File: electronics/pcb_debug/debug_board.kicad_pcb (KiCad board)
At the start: 2 copper layers, 40.9 x 30.6 mm, 11 parts, among them J1 SWD Device, J2 SWD Probe

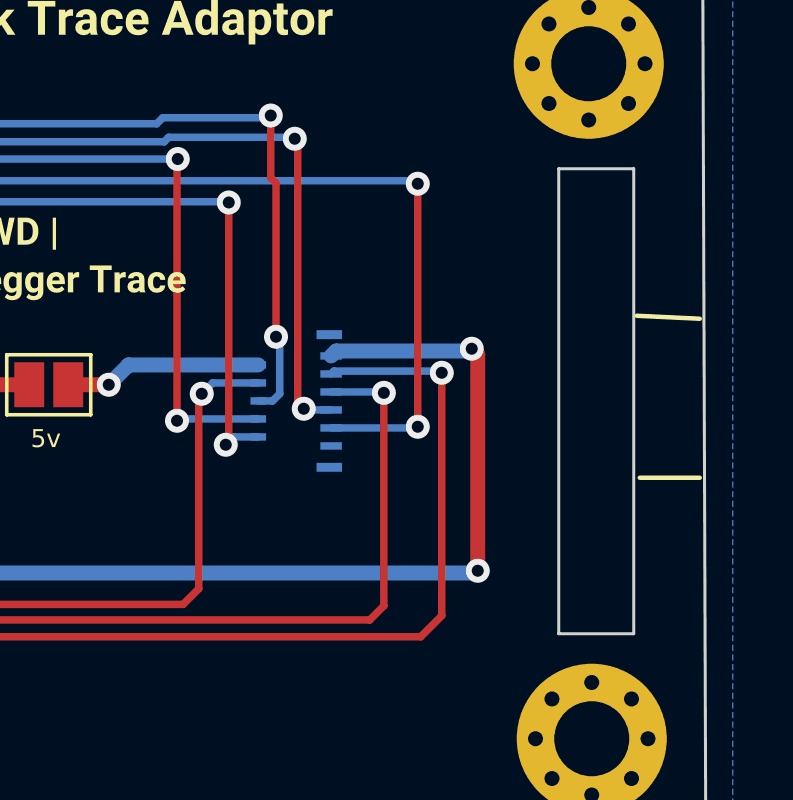
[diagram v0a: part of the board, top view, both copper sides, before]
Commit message: BOM update
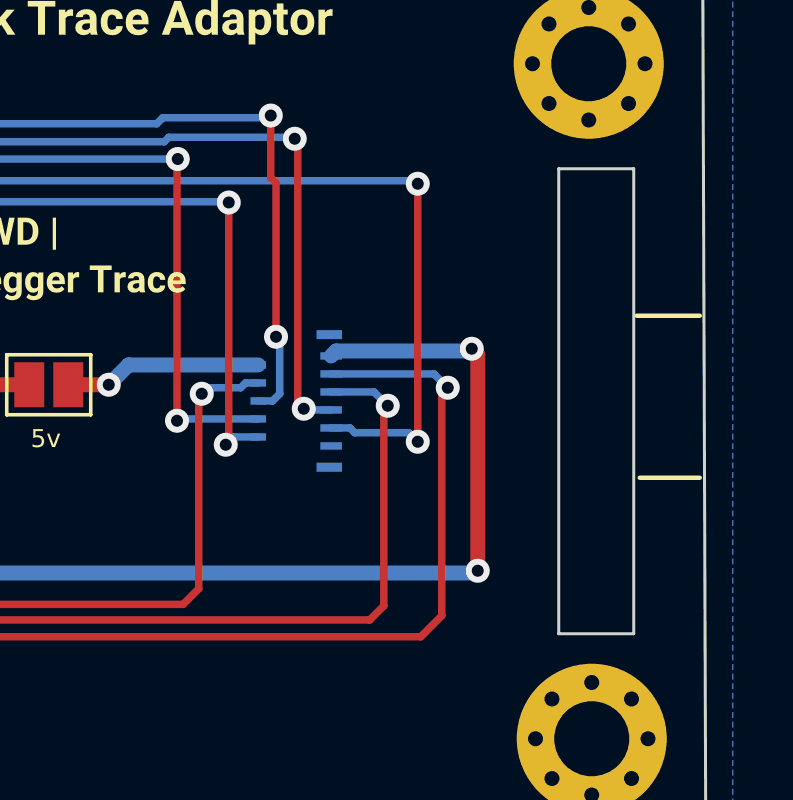
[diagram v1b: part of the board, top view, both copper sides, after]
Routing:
- net /TRACED2: track 33.9 -> 34.6 mm
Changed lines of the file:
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@@
   (gr_circle (center 94.6 65) (end 94.916228 65) (layer "F.SilkS") (width 0.15) (fill solid))
   (gr_rect (start 94 58.2) (end 94.9 60.4) (layer "F.SilkS") (width 0.15) (fill solid))
-  (gr_line (start 119.9 56.5) (end 117.8 56.4) (layer "F.SilkS") (width 0.15))
+  (gr_line (start 119.9 56.4) (end 117.8 56.4) (layer "F.SilkS") (width 0.15))
   (gr_line (start 119.9 61.8) (end 117.9 61.8) (layer "F.SilkS") (width 0.15))
   (gr_line (start 79.207107 44.907107) (end 79.2 73.5) (layer "Edge.Cuts") (width 0.1))
@@
   (segment (start 100.86 58.04) (end 100.2 58.7) (width 0.5) (layer "B.Cu") (net 2))
   (segment (start 105.1835 58.04) (end 100.86 58.04) (width 0.5) (layer "B.Cu") (net 2))
+  (segment (start 89.9 66.2) (end 89.9 60.4) (width 0.25) (layer "F.Cu") (net 3))
+  (segment (start 89.9 60.4) (end 90.405 59.895) (width 0.25) (layer "F.Cu") (net 3))
   (segment (start 90.8 67.1) (end 89.9 66.2) (width 0.25) (layer "F.Cu") (net 3))
-  (segment (start 111.3 58.3) (end 111.3 66.4) (width 0.25) (layer "F.Cu") (net 3))
-  (segment (start 89.9 60.4) (end 90.405 59.895) (width 0.25) (layer "F.Cu") (net 3))
+  (segment (start 111.3 59) (end 111.3 66.4) (width 0.25) (layer "F.Cu") (net 3))
+  (segment (start 111.5 58.8) (end 111.3 59) (width 0.25) (layer "F.Cu") (net 3))
+  (segment (start 111.3 66.4) (end 110.6 67.1) (width 0.25) (layer "F.Cu") (net 3))
   (segment (start 110.6 67.1) (end 90.8 67.1) (width 0.25) (layer "F.Cu") (net 3))
   (segment (start 90.405 59.895) (end 91.555 59.895) (width 0.25) (layer "F.Cu") (net 3))
-  (segment (start 111.3 66.4) (end 110.6 67.1) (width 0.25) (layer "F.Cu") (net 3))
-  (segment (start 89.9 66.2) (end 89.9 60.4) (width 0.25) (layer "F.Cu") (net 3))
-  (via (at 111.3 58.3) (size 0.8) (drill 0.4) (layers "F.Cu" "B.Cu") (net 3))
-  (segment (start 107.6135 58.34) (end 107.708011 58.245489) (width 0.25) (layer "B.Cu") (net 3))
-  (segment (start 107.708011 58.245489) (end 111.245489 58.245489) (width 0.25) (layer "B.Cu") (net 3))
-  (segment (start 111.245489 58.245489) (end 111.3 58.3) (width 0.25) (layer "B.Cu") (net 3))
+  (via (at 111.5 58.8) (size 0.8) (drill 0.4) (layers "F.Cu" "B.Cu") (net 3))
+  (segment (start 111.5 58.8) (end 111.04 58.34) (width 0.25) (layer "B.Cu") (net 3))
+  (segment (start 111.04 58.34) (end 107.6135 58.34) (width 0.25) (layer "B.Cu") (net 3))
   (segment (start 91.92 66.02) (end 91.555 65.655) (width 0.25) (layer "F.Cu") (net 4))
   (segment (start 103.3 59) (end 103.2 59.1) (width 0.25) (layer "F.Cu") (net 4))
@@
   (segment (start 91.555 65.655) (end 91.555 64.975) (width 0.25) (layer "F.Cu") (net 4))
   (via (at 103.3 59) (size 0.8) (drill 0.4) (layers "F.Cu" "B.Cu") (net 4))
-  (segment (start 103.66 58.64) (end 105.1835 58.64) (width 0.25) (layer "B.Cu") (net 4))
-  (segment (start 103.3 59) (end 103.66 58.64) (width 0.25) (layer "B.Cu") (net 4))
+  (segment (start 103.5 58.8) (end 104.598989 58.8) (width 0.25) (layer "B.Cu") (net 4))
+  (segment (start 104.758989 58.64) (end 105.1835 58.64) (width 0.25) (layer "B.Cu") (net 4))
+  (segment (start 103.3 59) (end 103.5 58.8) (width 0.25) (layer "B.Cu") (net 4))
+  (segment (start 104.598989 58.8) (end 104.758989 58.64) (width 0.25) (layer "B.Cu") (net 4))
+  (segment (start 109.5 59.4) (end 109.37 59.53) (width 0.25) (layer "F.Cu") (net 5))
+  (segment (start 91.17952 66.53952) (end 90.46 65.82) (width 0.25) (layer "F.Cu") (net 5))
+  (segment (start 109.37 66.07) (end 108.90048 66.53952) (width 0.25) (layer "F.Cu") (net 5))
+  (segment (start 109.37 59.53) (end 109.37 66.07) (width 0.25) (layer "F.Cu") (net 5))
   (segment (start 90.46 64.19) (end 90.945 63.705) (width 0.25) (layer "F.Cu") (net 5))
-  (segment (start 91.17952 66.53952) (end 90.46 65.82) (width 0.25) (layer "F.Cu") (net 5))
-  (segment (start 109.37 58.97) (end 109.37 66.07) (width 0.25) (layer "F.Cu") (net 5))
   (segment (start 108.90048 66.53952) (end 91.17952 66.53952) (width 0.25) (layer "F.Cu") (net 5))
-  (segment (start 109.37 66.07) (end 108.90048 66.53952) (width 0.25) (layer "F.Cu") (net 5))
+  (segment (start 90.46 65.82) (end 90.46 64.19) (width 0.25) (layer "F.Cu") (net 5))
   (segment (start 90.945 63.705) (end 91.555 63.705) (width 0.25) (layer "F.Cu") (net 5))
-  (segment (start 90.46 65.82) (end 90.46 64.19) (width 0.25) (layer "F.Cu") (net 5))
-  (via (at 109.37 58.97) (size 0.8) (drill 0.4) (layers "F.Cu" "B.Cu") (net 5))
-  (segment (start 107.6135 58.94) (end 109.34 58.94) (width 0.25) (layer "B.Cu") (net 5))
-  (segment (start 109.34 58.94) (end 109.37 58.97) (width 0.25) (layer "B.Cu") (net 5))
+  (via (at 109.5 59.4) (size 0.8) (drill 0.4) (layers "F.Cu" "B.Cu") (net 5))
+  (segment (start 109.04 58.94) (end 107.6135 58.94) (width 0.25) (layer "B.Cu") (net 5))
+  (segment (start 109.5 59.4) (end 109.04 58.94) (width 0.25) (layer "B.Cu") (net 5))
   (segment (start 89.325 58.625) (end 91.555 58.625) (width 0.25) (layer "F.Cu") (net 6))
   (segment (start 105.6 49.726489) (end 105.6 51.8) (width 0.25) (layer "F.Cu") (net 6))
@@
   (segment (start 90.799913 51.175489) (end 102.499989 51.175489) (width 0.25) (layer "B.Cu") (net 8))
   (segment (start 91.100011 51.899989) (end 90.64952 52.35048) (width 0.25) (layer "F.Cu") (net 9))
-  (segment (start 110.5 52) (end 110.5 60.1) (width 0.25) (layer "F.Cu") (net 9))
   (segment (start 90.64952 52.35048) (end 90.64952 53.90952) (width 0.25) (layer "F.Cu") (net 9))
+  (segment (start 110.5 52) (end 110.5 60.6) (width 0.25) (layer "F.Cu") (net 9))
   (segment (start 91.452741 51.899989) (end 91.100011 51.899989) (width 0.25) (layer "F.Cu") (net 9))
   (segment (start 90.64952 53.90952) (end 91.555 54.815) (width 0.25) (layer "F.Cu") (net 9))
-  (via (at 110.5 60.1) (size 0.8) (drill 0.4) (layers "F.Cu" "B.Cu") (net 9))
+  (via (at 110.5 60.6) (size 0.8) (drill 0.4) (layers "F.Cu" "B.Cu") (net 9))
   (via (at 91.452741 51.899989) (size 0.8) (drill 0.4) (layers "F.Cu" "B.Cu") (net 9))
   (via (at 110.5 52) (size 0.8) (drill 0.4) (layers "F.Cu" "B.Cu") (net 9))
+  (segment (start 110.5 60.6) (end 110.2 60.3) (width 0.25) (layer "B.Cu") (net 9))
   (segment (start 110.4 51.9) (end 110.5 52) (width 0.25) (layer "B.Cu") (net 9))
-  (segment (start 110.46 60.14) (end 107.6135 60.14) (width 0.25) (layer "B.Cu") (net 9))
   (segment (start 91.452741 51.899989) (end 91.452752 51.9) (width 0.25) (layer "B.Cu") (net 9))
   (segment (start 91.452752 51.9) (end 110.4 51.9) (width 0.25) (layer "B.Cu") (net 9))
-  (segment (start 110.5 60.1) (end 110.46 60.14) (width 0.25) (layer "B.Cu") (net 9))
+  (segment (start 108.24 60.14) (end 107.6135 60.14) (width 0.25) (layer "B.Cu") (net 9))
+  (segment (start 108.4 60.3) (end 108.24 60.14) (width 0.25) (layer "B.Cu") (net 9))
+  (segment (start 110.2 60.3) (end 108.4 60.3) (width 0.25) (layer "B.Cu") (net 9))
   (segment (start 104.2 52.6245) (end 104.2 60.6) (width 0.25) (layer "F.Cu") (net 10))
   (segment (start 94.6 52.6245) (end 94.4755 52.5) (width 0.25) (layer "F.Cu") (net 10))

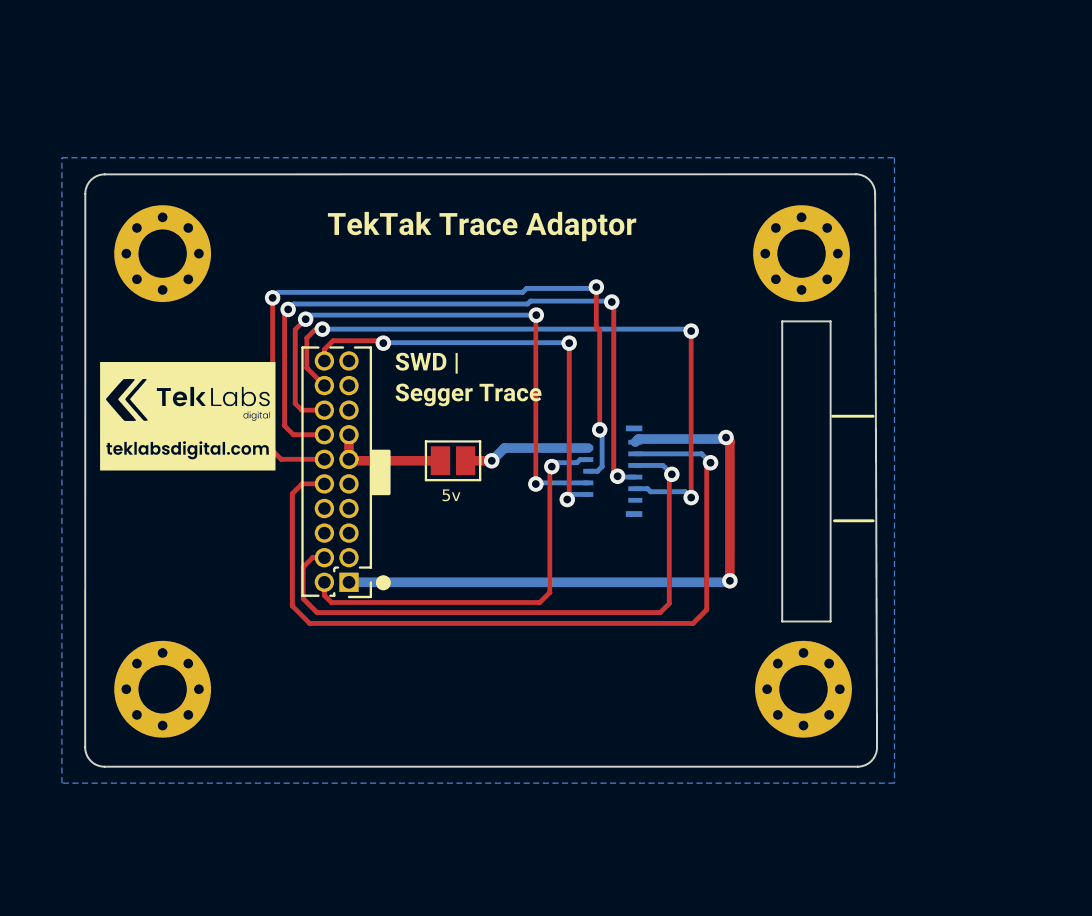
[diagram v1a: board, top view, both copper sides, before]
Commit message: Hardware and Firmware udpates
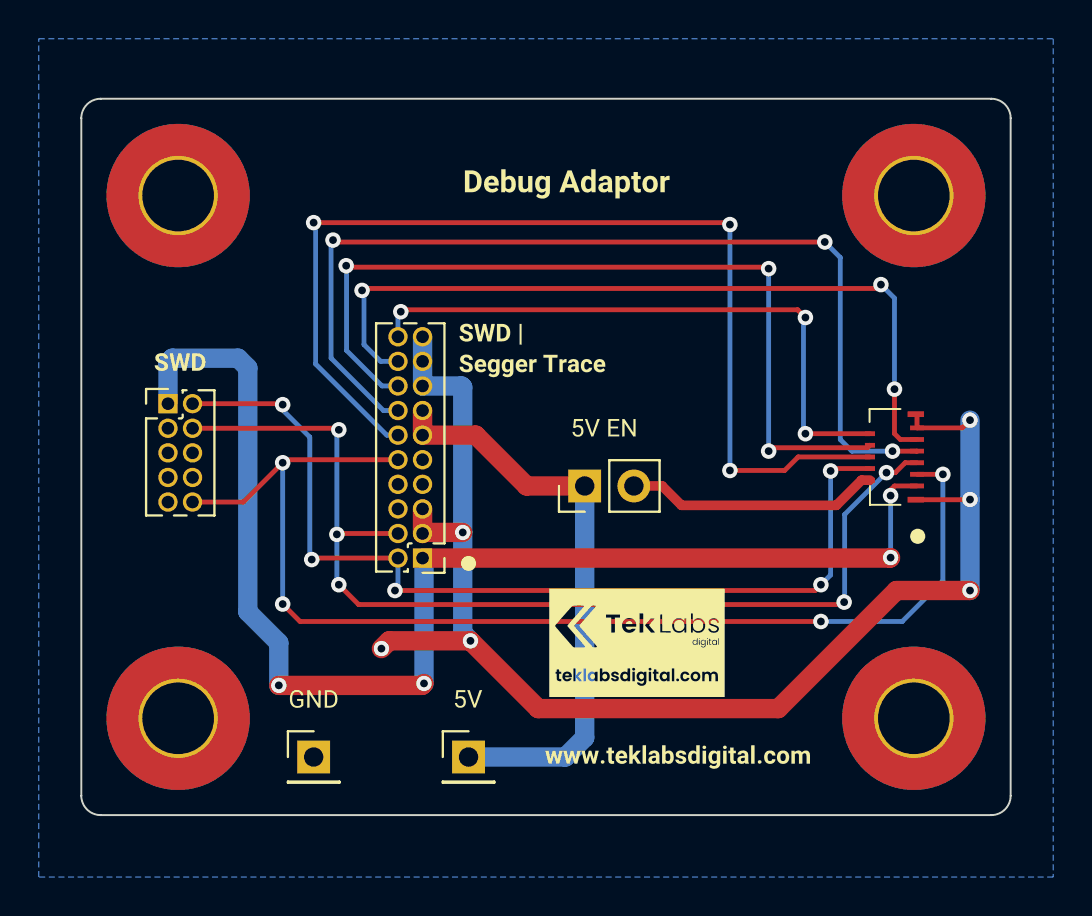
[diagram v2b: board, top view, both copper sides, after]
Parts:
- removed kibuzzard-647579C7: G***, kibuzzard-647579C7
- removed kibuzzard-64757A48: G***, kibuzzard-64757A48
- added J3: SWD Debug, Connector_PinHeader_1.27mm:PinHeader_2x05_P1.27mm_Vertical, F.Cu at (83.5, 55.8)
- added J4: 5V, Connector_PinHeader_2.54mm:PinHeader_1x01_P2.54mm_Vertical, F.Cu at (99.0, 74.0)
- added J5: GND, Connector_PinHeader_2.54mm:PinHeader_1x01_P2.54mm_Vertical, F.Cu at (91.0, 74.0)
- added kibuzzard-64C06064: G***, kibuzzard-64C06064, F.Cu at (84.1, 53.6)
- added kibuzzard-64C06F13: G***, kibuzzard-64C06F13, F.Cu at (109.8, 74.0)
- added kibuzzard-64C06F53: G***, kibuzzard-64C06F53, F.Cu at (104.1, 44.4)
- added kibuzzard-64C0828D: G***, kibuzzard-64C0828D, F.Cu at (91.0, 71.0)
- added kibuzzard-64C082C5: G***, kibuzzard-64C082C5, F.Cu at (99.0, 71.0)
- added kibuzzard-64C08352: G***, kibuzzard-64C08352, F.Cu at (106.0, 57.0)
- H1, H2, H3, H4: footprint MountingHole:MountingHole_2.5mm_Pad_Via -> MountingHole:MountingHole_3.7mm_Pad_TopBottom
- J1: value SWD Device -> SWD Trace; moved to F.Cu
- J2: value SWD Probe -> SWD Trace J Trace
- JP1: footprint Jumper:SolderJumper-2_P1.3mm_Open_Pad1.0x1.5mm -> Connector_PinHeader_2.54mm:PinHeader_1x02_P2.54mm_Vertical
- moved G*** 26.0 mm to (107.7, 68.1)
- moved J1 15.0 mm to (119.7, 57.0), turned to 90 degrees
- moved JP1 6.92 mm to (105.0, 60.0), turned to 90 degrees
- moved H3 6.53 mm to (122.0, 45.0)
- moved H1 5.89 mm to (122.0, 72.0)
- moved J2 4.00 mm to (96.6, 63.7)
- moved kibuzzard-64757A2A 3.62 mm to (102.3, 53.0)
- moved H4 3.10 mm to (84.0, 45.0)
- moved H2 1.70 mm to (84.0, 72.0)
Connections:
- JP1 pad 1: Net-(J1-Pad2) -> +5V
- JP1 pad 2: +5V -> Net-(J1-Pad2)
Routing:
- net GND: track 0.00 -> 71.1 mm, vias 0 -> 6
- net VDD: track 32.0 -> 66.8 mm, vias 2 -> 4
- net /SWDIO: track 21.3 -> 49.8 mm, vias 1 -> 5
- net +5V: track 6.03 -> 30.1 mm
- net /SWCLK: track 31.1 -> 54.8 mm, vias 1 -> 5
- net /~{nRESET}: track 41.5 -> 61.0 mm, vias 1 -> 4
- net /TRACECLK: track 37.9 -> 54.9 mm
- net /TRACED0: track 35.3 -> 50.9 mm
- net /TRACED1: track 29.7 -> 44.5 mm
- net /TRACED3: track 22.8 -> 31.9 mm
- net /TRACED2: track 34.6 -> 41.2 mm
- net Net-(J1-Pad2): track 6.61 -> 13.1 mm, vias 1 -> 0
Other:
- board size 40.9 x 30.6 mm -> 48 x 37 mm
- board text removed: "5v"
